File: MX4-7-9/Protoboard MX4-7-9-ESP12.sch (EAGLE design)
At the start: 52 parts

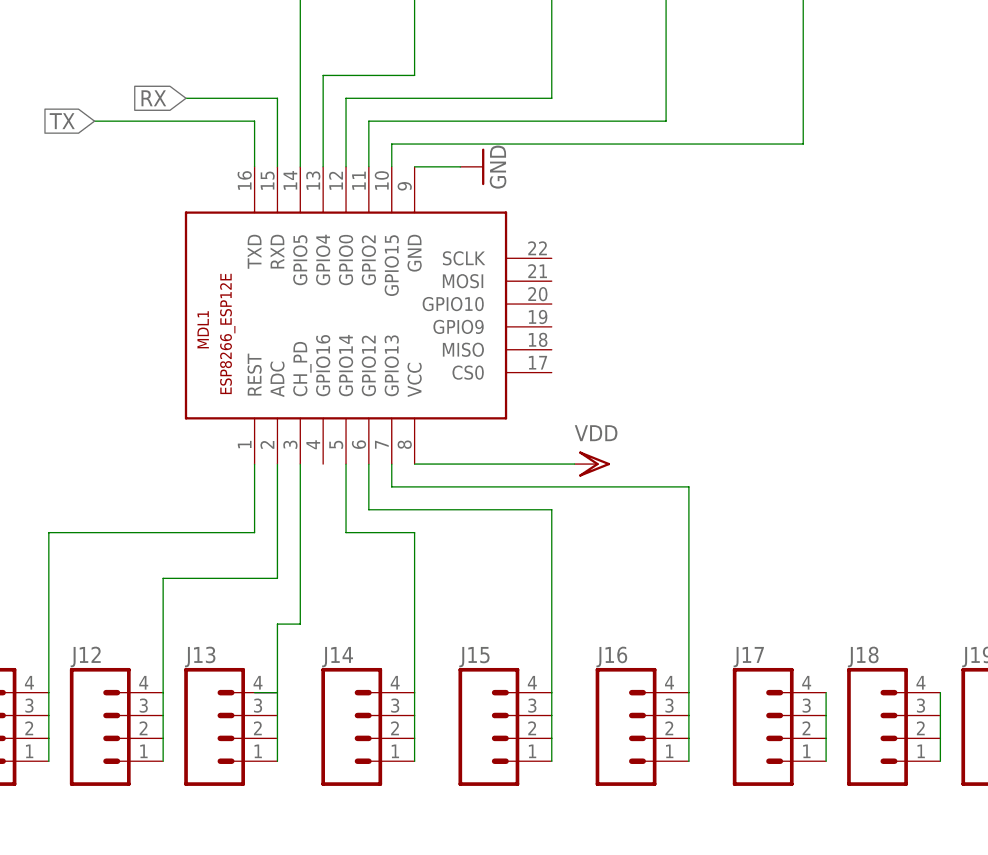
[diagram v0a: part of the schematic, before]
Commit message: Update esp component and usb
test
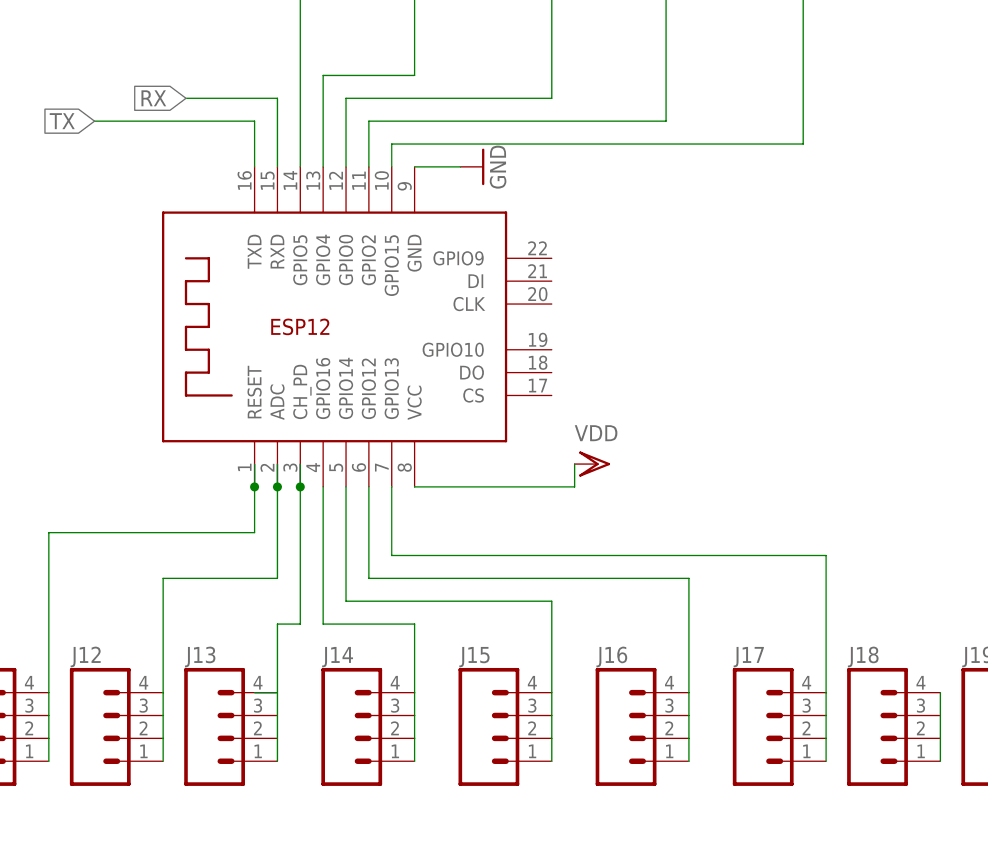
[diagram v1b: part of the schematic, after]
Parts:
- removed MDL1: (no value), ESP8266-ESP12E:ESP8266-12EESP8266-ESP12E
- added X1: ESP-12E, microbuilder:ESP-12E
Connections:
- net GND: now also X1.GND; no longer MDL1.GND
- net N$10: now also X1.GPIO4; no longer MDL1.GPIO4
- net N$11: now also X1.GPIO0; no longer MDL1.GPIO0
- net N$12: now also X1.GPIO2; no longer MDL1.GPIO2
- net N$13: now also X1.GPIO15; no longer MDL1.GPIO15
- net N$26: now also X1.GPIO16; no longer MDL1.GPIO14
- net N$34: now also X1.GPIO13
- net N$50: now also X1.RESET; no longer MDL1.REST
- net N$51: now also X1.ADC; no longer MDL1.ADC
- net N$52: now also X1.CH_PD; no longer MDL1.CH_PD
- net N$55: now also X1.GPIO14; no longer MDL1.GPIO12
- net N$56: now also X1.GPIO12; no longer MDL1.GPIO13
- net N$9: now also X1.GPIO5; no longer MDL1.GPIO5
- net RX: now also X1.RXD; no longer MDL1.RXD
- net TX: now also X1.TXD; no longer MDL1.TXD
- net VDD: now also X1.VCC; no longer MDL1.VCC
